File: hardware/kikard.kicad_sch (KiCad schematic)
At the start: 73 parts, among them Q1 WNM3013-3/TR, Q2 WNM3013-3/TR, SW1 K2-6639SP-C4SC-04, SW2 K2-6639SP-C4SC-04, SW3 K2-6639SP-C4SC-04, SW4 HX TS-1088-AR02016, U1 NRF52840-QIAA-R, U2 ST25R3916-AQWT, Y1 27MHz, Y2 32MHz, Y3 32.768kHz

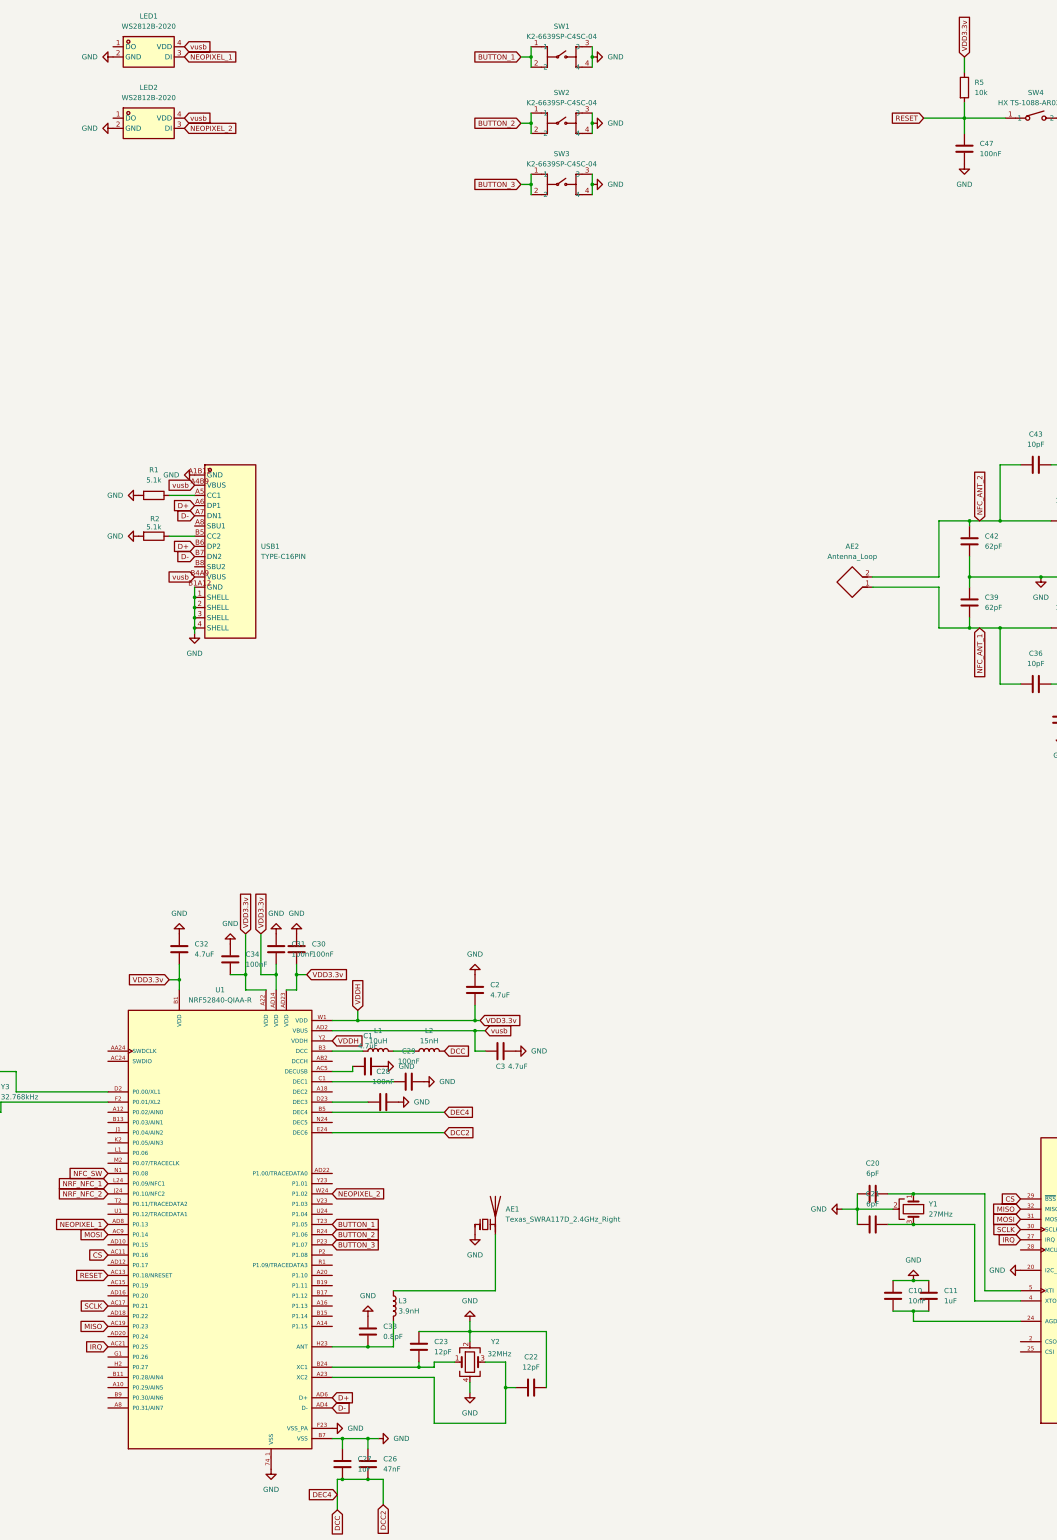
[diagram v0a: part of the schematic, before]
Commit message: 7-18-25
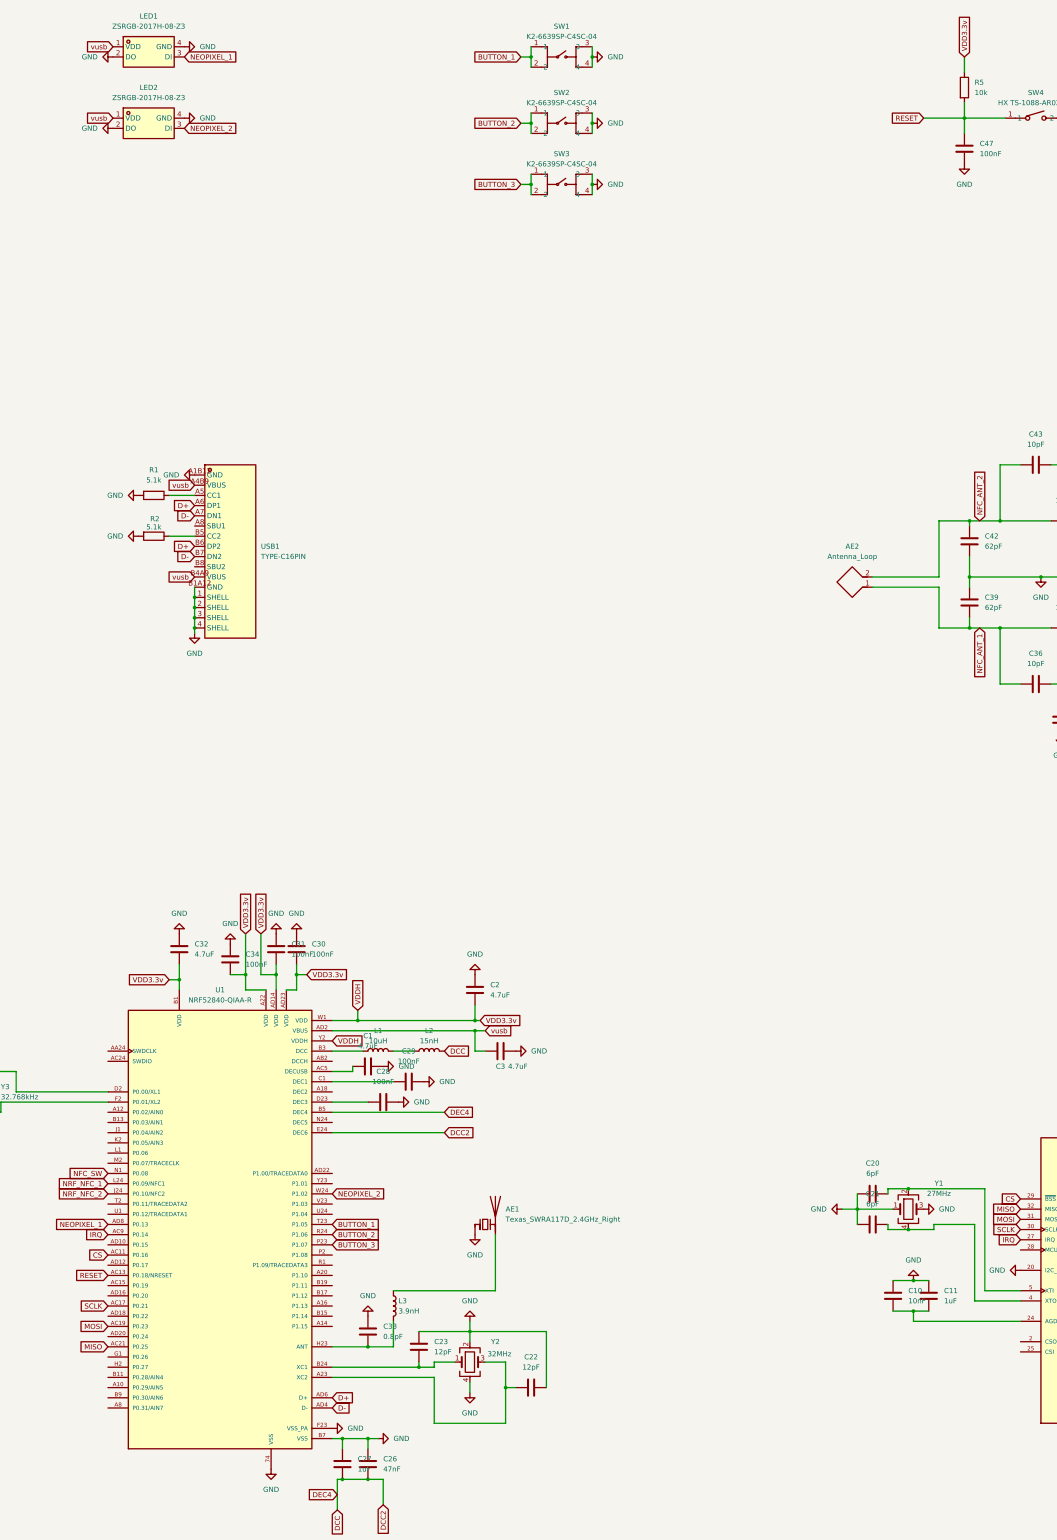
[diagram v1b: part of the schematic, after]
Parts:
- removed Y1: 27MHz, extra-symbols-footprints:CRYSTAL-SMD_4P-L2.0-W1.6-BL-B, symbol Device:Crystal_GND2
- added Y1: 27MHz, extra-symbols-footprints:CRYSTAL-SMD_4P-L2.0-W1.6-BL-B, symbol Device:Crystal_GND24
- L3: footprint extra-symbols-footprints:R0402 -> extra-symbols-footprints:L0402
- LED1, LED2: value WS2812B-2020 -> ZSRGB-2017H-08-Z3; footprint extra-symbols-footprints:LED-SMD_4P-L2.0-W2.0-TL_WS2812B-2020 -> extra-symbols-footprints:LED-SMD_4P-L2.0-W1.8-P0.90_XGM-S0807RGB; symbol WS2812B-2020:WS2812B-2020 -> rgbled:ZSRGB-2017H-08-Z3; LCSC Part C965555 -> C7497245
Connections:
- net GND: now also LED1.4 (GND), LED2.4 (GND), U1.74 (VSS), Y1.1, Y1.3; no longer U1.74_1 (VSS)
- net IRQ: now also U1.AC9 (P0.14); no longer U1.AC21 (P0.25)
- net MISO: now also U1.AC21 (P0.25); no longer U1.AC19 (P0.23)
- net MOSI: now also U1.AC19 (P0.23); no longer U1.AC9 (P0.14)
- net vusb: now also LED1.1 (VDD), LED2.1 (VDD); no longer LED1.4 (VDD), LED2.4 (VDD)
- net at C20.2, U2.5 (XTI): now also Y1.2
- net at C21.2, U2.4 (XTO): now also Y1.4
